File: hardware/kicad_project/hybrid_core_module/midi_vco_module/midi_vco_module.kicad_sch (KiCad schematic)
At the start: 38 parts, among them J1 AudioJack2_SwitchT, J2 Screw_Terminal_01x08, J3 AudioJack2_SwitchT, J4 AudioJack2_SwitchT, J5 AudioJack2_SwitchT, J6 AudioJack2_SwitchT, J8 AudioJack2_SwitchT, Q13 2N7002, Q7 2N7002, SW2 SW_Rotary_1x4_MP, SW3 SW_Rotary_1x4_MP, SW6 SW_SPDT

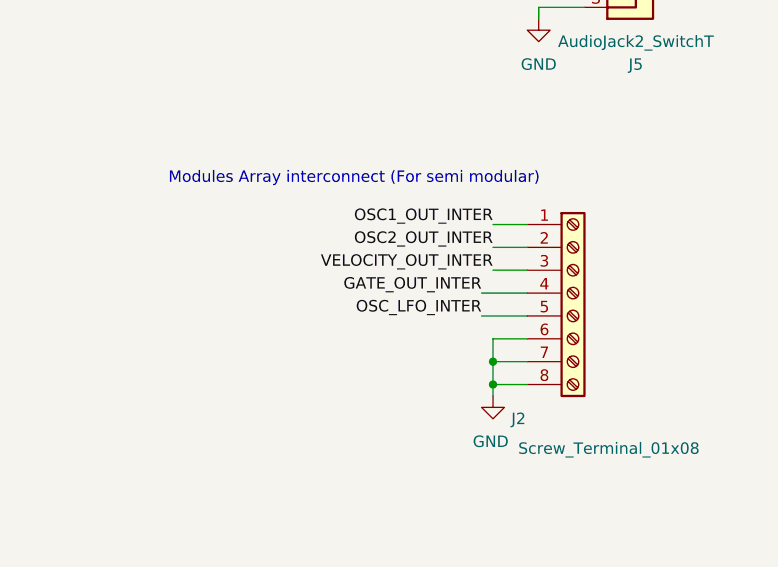
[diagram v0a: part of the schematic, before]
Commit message: routing continued.
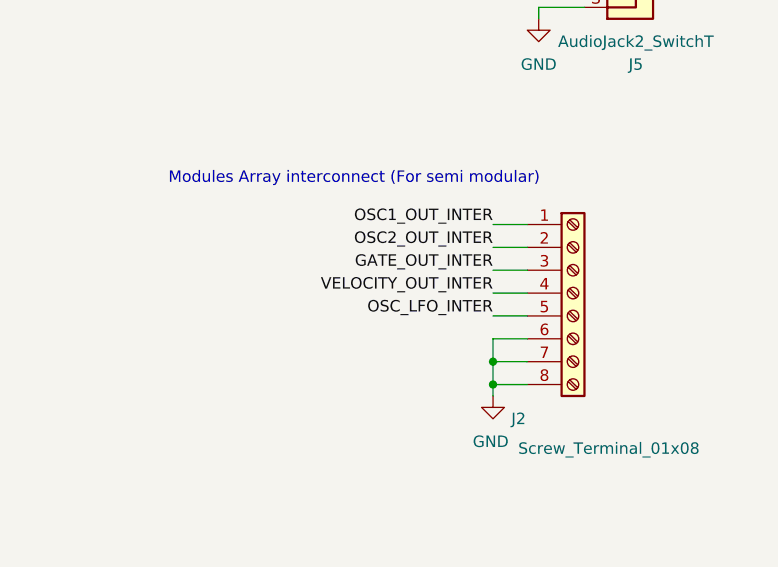
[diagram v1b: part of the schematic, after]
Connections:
- net GATE_OUT_INTER: now also J2.3 (Pin_3); no longer J2.4 (Pin_4)
- net VELOCITY_OUT_INTER: now also J2.4 (Pin_4); no longer J2.3 (Pin_3)
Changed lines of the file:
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@@
 	(wire
 		(pts
-			(xy 255.27 144.78) (xy 260.35 144.78)
+			(xy 256.54 144.78) (xy 260.35 144.78)
 		)
 		(stroke
@@
 	(wire
 		(pts
-			(xy 255.27 147.32) (xy 260.35 147.32)
+			(xy 256.54 147.32) (xy 260.35 147.32)
 		)
 		(stroke
@@
 		)
 	)
-	(label "OSC2_OUT_INTER"
-		(at 256.54 139.7 180)
-		(effects
-			(font
-				(size 1.27 1.27)
-			)
-			(justify right bottom)
-		)
-	)
 	(label "CALIBATION_MODE"
 		(at 92.71 180.34 180)
@@
 	)
 	(label "VELOCITY_OUT_INTER"
+		(at 256.54 144.78 180)
+		(effects
+			(font
+				(size 1.27 1.27)
+			)
+			(justify right bottom)
+		)
+	)
+	(label "VELOCITY_OUT_INTER"
 		(at 265.43 92.71 180)
 		(effects
@@
 		)
 	)
-	(label "OSC_LFO_INTER"
-		(at 255.27 147.32 180)
+	(label "OSC2_OUT_INTER"
+		(at 256.54 139.7 180)
 		(effects
 			(font
@@
 		)
 	)
-	(label "VELOCITY_OUT_INTER"
-		(at 256.54 142.24 180)
-		(effects
-			(font
-				(size 1.27 1.27)
-			)
-			(justify right bottom)
-		)
-	)
 	(label "VELOCITY_OUT"
 		(at 262.89 95.25 180)
@@
 		)
 	)
-	(label "GATE_OUT"
-		(at 259.08 110.49 180)
+	(label "OSC_LFO_INTER"
+		(at 256.54 147.32 180)
 		(effects
 			(font
@@
 		)
 	)
-	(label "OSC1_OUT_INTER"
-		(at 267.97 33.02 180)
+	(label "GATE_OUT_INTER"
+		(at 256.54 142.24 180)
 		(effects
 			(font
@@
 		)
 	)
-	(label "GATE_OUT_INTER"
-		(at 255.27 144.78 180)
+	(label "GATE_OUT"
+		(at 259.08 110.49 180)
+		(effects
+			(font
+				(size 1.27 1.27)
+			)
+			(justify right bottom)
+		)
+	)
+	(label "OSC1_OUT_INTER"
+		(at 267.97 33.02 180)
 		(effects
 			(font
@@
 		)
 		(instances
-			(project ""
+			(project "midi_vco_module"
 				(path "/3378c2b5-f4b3-47f0-8cdf-dba4991b82b5"
 					(reference "J2")
